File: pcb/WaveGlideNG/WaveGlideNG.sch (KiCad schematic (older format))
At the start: 22 parts, among them J1 feather long, J2 feather short

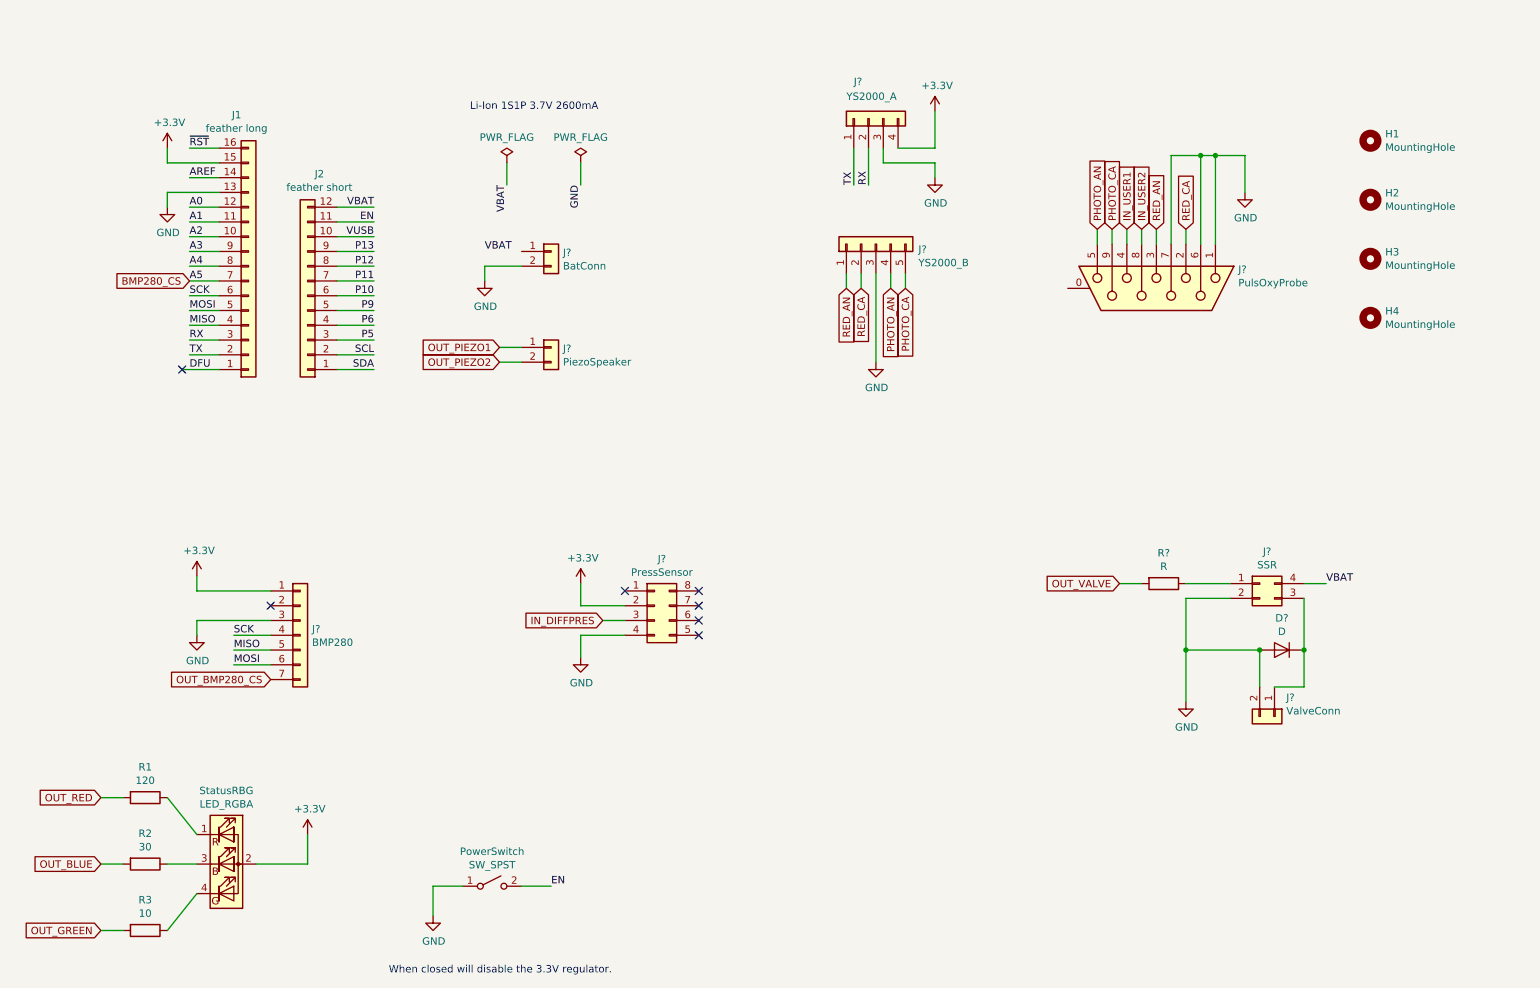
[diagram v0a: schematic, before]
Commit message: footprints
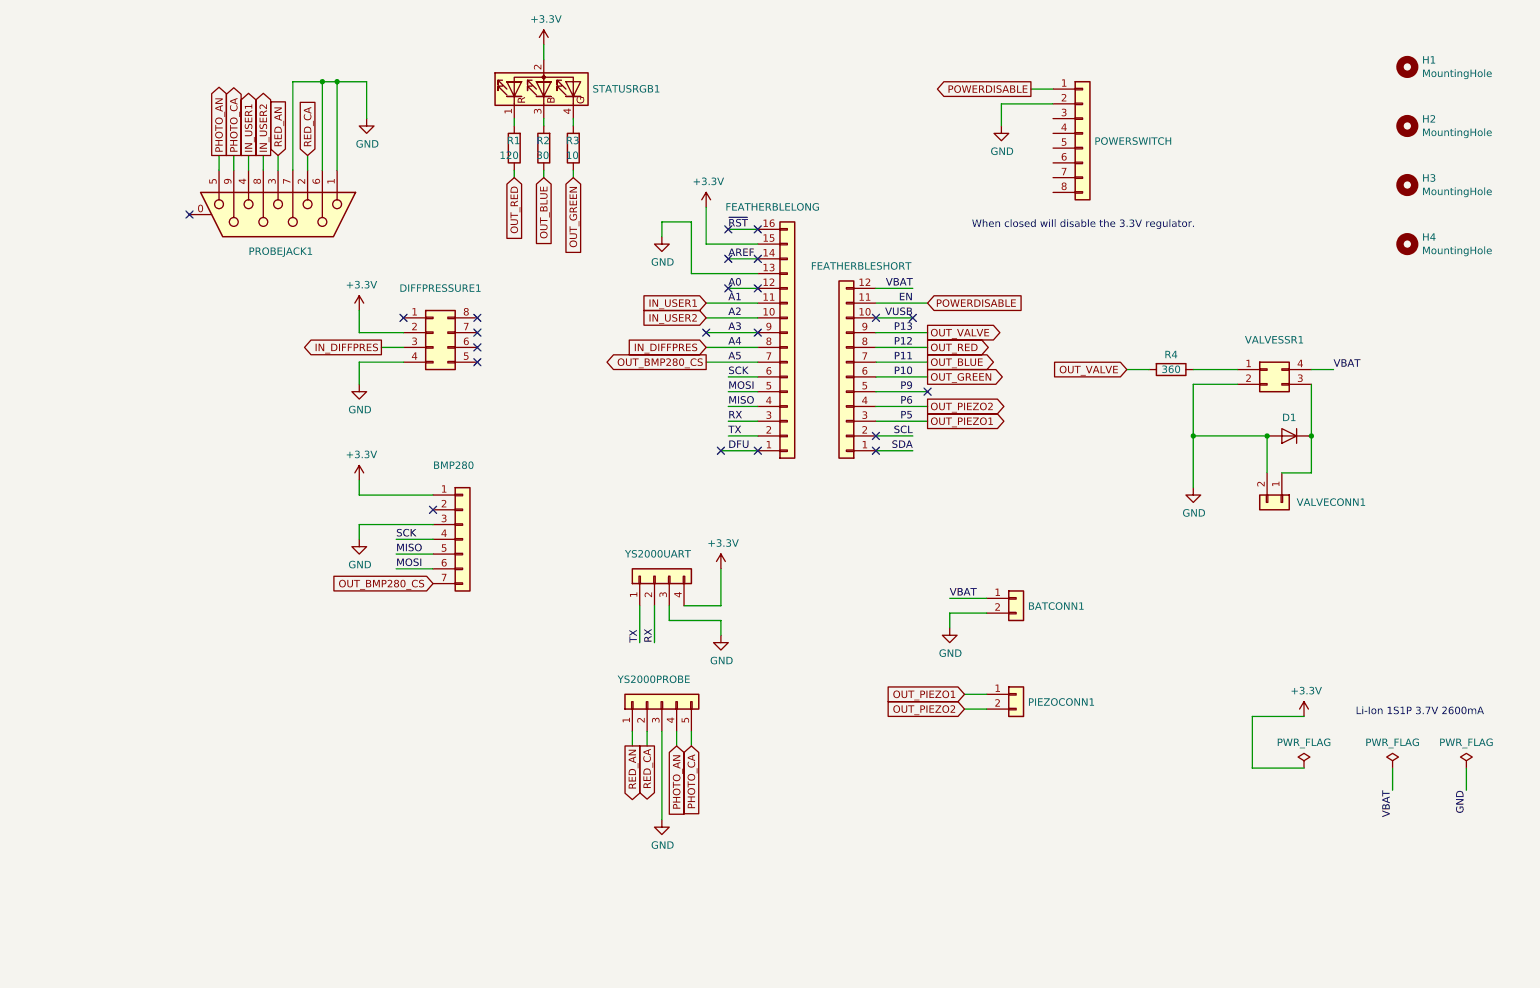
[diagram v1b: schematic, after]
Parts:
- removed PowerSwitch: SW_SPST, symbol Switch:SW_SPST
- added POWERSWITCH1: POWERSWITCH, WaveGlideNG:TE_Switch, symbol Connector_Generic:Conn_01x08
- BATCONN1: renamed from J?; value BatConn -> BATCONN; footprint (none) -> Pin_Headers:Pin_Header_Straight_1x02_Pitch2.54mm
- BMP280: renamed from J?; footprint (none) -> Pin_Headers:Pin_Header_Straight_1x07_Pitch2.54mm
- D1: renamed from D?; footprint (none) -> Diodes_ThroughHole:D_5KPW_P12.70mm_Horizontal
- DIFFPRESSURE1: renamed from J?; footprint (none) -> WaveGlideNG:DIFFPRESS
- FEATHERBLELONG1: renamed from J1; value feather long -> FEATHERBLELONG
- FEATHERBLESHORT1: renamed from J2; value feather short -> FEATHERBLESHORT
- PIEZOCONN1: renamed from J?; value PiezoSpeaker -> PIEZOCONN; footprint (none) -> WaveGlideNG:PIEZO
- PROBEJACK1: renamed from J?; value PulsOxyProbe -> PROBEJACK; footprint (none) -> WaveGlideNG:DB9HARTING
- R1, R2, R3: footprint (none) -> Resistors_ThroughHole:R_Axial_Power_L48.0mm_W12.5mm_P7.62mm_Vertical
- R4: renamed from R?; value R -> 360; footprint (none) -> Resistors_ThroughHole:R_Axial_Power_L48.0mm_W12.5mm_P7.62mm_Vertical
- STATUSRGB1: renamed from StatusRBG; value LED_RGBA -> STATUSRGB; footprint (none) -> WaveGlideNG:RGBA_5mm
- VALVECONN1: renamed from J?; value ValveConn -> VALVECONN; footprint (none) -> Pin_Headers:Pin_Header_Straight_1x02_Pitch2.54mm
- VALVESSR1: renamed from J?; value SSR -> VALVESSR; footprint (none) -> Pin_Headers:Pin_Header_Straight_1x02_Pitch2.54mm
- YS2000PROBE1: renamed from J?; value YS2000_B -> YS2000PROBE; footprint (none) -> Pin_Headers:Pin_Header_Straight_1x05_Pitch2.54mm
- YS2000UART1: renamed from J?; value YS2000_A -> YS2000UART; footprint (none) -> Pin_Headers:Pin_Header_Straight_1x04_Pitch2.54mm
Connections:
- net A1 is gone; now on net IN_USER1: FEATHERBLELONG1.11 (Pin_11)
- net A2 is gone; now on net IN_USER2: FEATHERBLELONG1.10 (Pin_10)
- net A4 is gone; now on net IN_DIFFPRES: FEATHERBLELONG1.8 (Pin_8)
- net BMP280_CS is gone; now on net OUT_BMP280_CS: FEATHERBLELONG1.7 (Pin_7)
- net P10 is gone; now on net OUT_GREEN: FEATHERBLESHORT1.6 (Pin_6)
- net P11 is gone; now on net OUT_BLUE: FEATHERBLESHORT1.7 (Pin_7)
- net P12 is gone; now on net OUT_RED: FEATHERBLESHORT1.8 (Pin_8)
- net P13 is gone; now on net OUT_VALVE: FEATHERBLESHORT1.9 (Pin_9)
- net P5 is gone; now on net OUT_PIEZO1: FEATHERBLESHORT1.3 (Pin_3)
- net P6 is gone; now on net OUT_PIEZO2: FEATHERBLESHORT1.4 (Pin_4)
- net GND: now also POWERSWITCH1.2 (Pin_2)
- net OUT_BLUE: now also R2.1; no longer R2.2
- net OUT_GREEN: now also R3.1; no longer R3.2
- net OUT_RED: now also R1.1; no longer R1.2
- net VBAT: now also BATCONN1.1 (Pin_1)
- net at STATUSRGB1.1 (RK): now also R1.2; no longer R1.1
- net at STATUSRGB1.3 (BK): now also R2.2; no longer R2.1
- net at STATUSRGB1.4 (GB): now also R3.2; no longer R3.1
- net EN renamed POWERDISABLE
- net POWERDISABLE: now also POWERSWITCH1.1 (Pin_1)
- no-connect marks 7 -> 22
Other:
- moved on the sheet: BATCONN1, BMP280, D1, DIFFPRESSURE1, H1, H2, H3, H4, PIEZOCONN1, PROBEJACK1, R1, R2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
